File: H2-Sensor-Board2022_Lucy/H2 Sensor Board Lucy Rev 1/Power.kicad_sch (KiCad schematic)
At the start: 42 parts, among them J2 Conn_02x03_Top_Bottom, Q1 NMOS, U3 AZ1117H-5.0, U4 TPS2596, U6 AZ1117EH-3.3

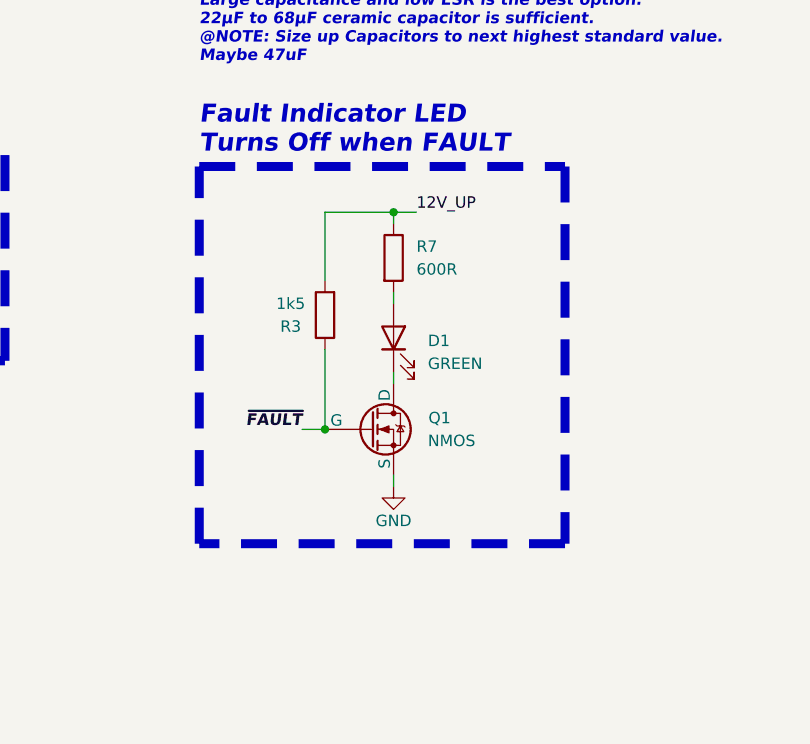
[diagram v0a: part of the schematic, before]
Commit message: fixzed some stuffs
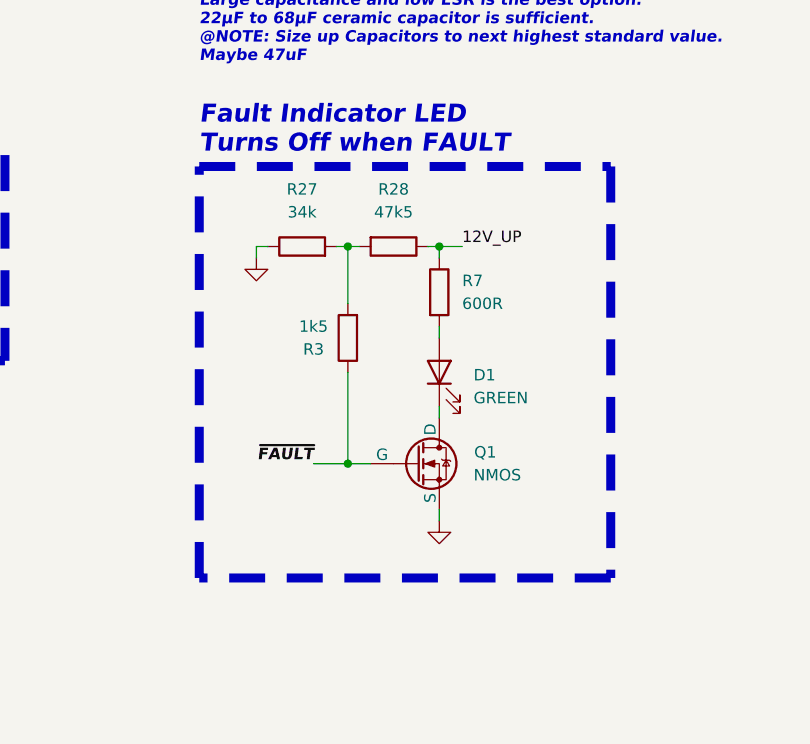
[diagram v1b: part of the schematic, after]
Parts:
- added R27: 34k, Resistor_SMD:R_0603_1608Metric, symbol Device:R
- added R28: 47k5, Resistor_SMD:R_0603_1608Metric, symbol Device:R
- R3: footprint Resistor_SMD:R_0805_2012Metric -> Resistor_SMD:R_0603_1608Metric
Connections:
- net 12V_UP: now also R28.1; no longer R3.2
- net GND: now also R27.1
- new net: R27.2, R28.2, R3.2
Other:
- moved on the sheet: D1, Q1, R3, R7

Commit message: Fixed some stuffs
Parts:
- C15, C18: JLCPCB Part#(Optional) (none) -> C1525
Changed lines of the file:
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@@
+      (effects (font (size 1.27 1.27)) hide)
+    )
+    (property "JLCPCB Part#(Optional)" "C1525" (at 142.24 48.26 0)
       (effects (font (size 1.27 1.27)) hide)
     )
@@
       (effects (font (size 1.27 1.27)) hide)
     )
+    (property "JLCPCB Part#(Optional)" "C1525" (at 99.06 48.26 0)
+      (effects (font (size 1.27 1.27)) hide)
+    )
